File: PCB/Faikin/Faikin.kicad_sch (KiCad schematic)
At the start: 30 parts, among them J1 1x5, J2 TC2030-USB-NL-DS, J3 Reset, Q1 BSS138PS, U2 ESP32-S3-MINI-1, U3 MD8942

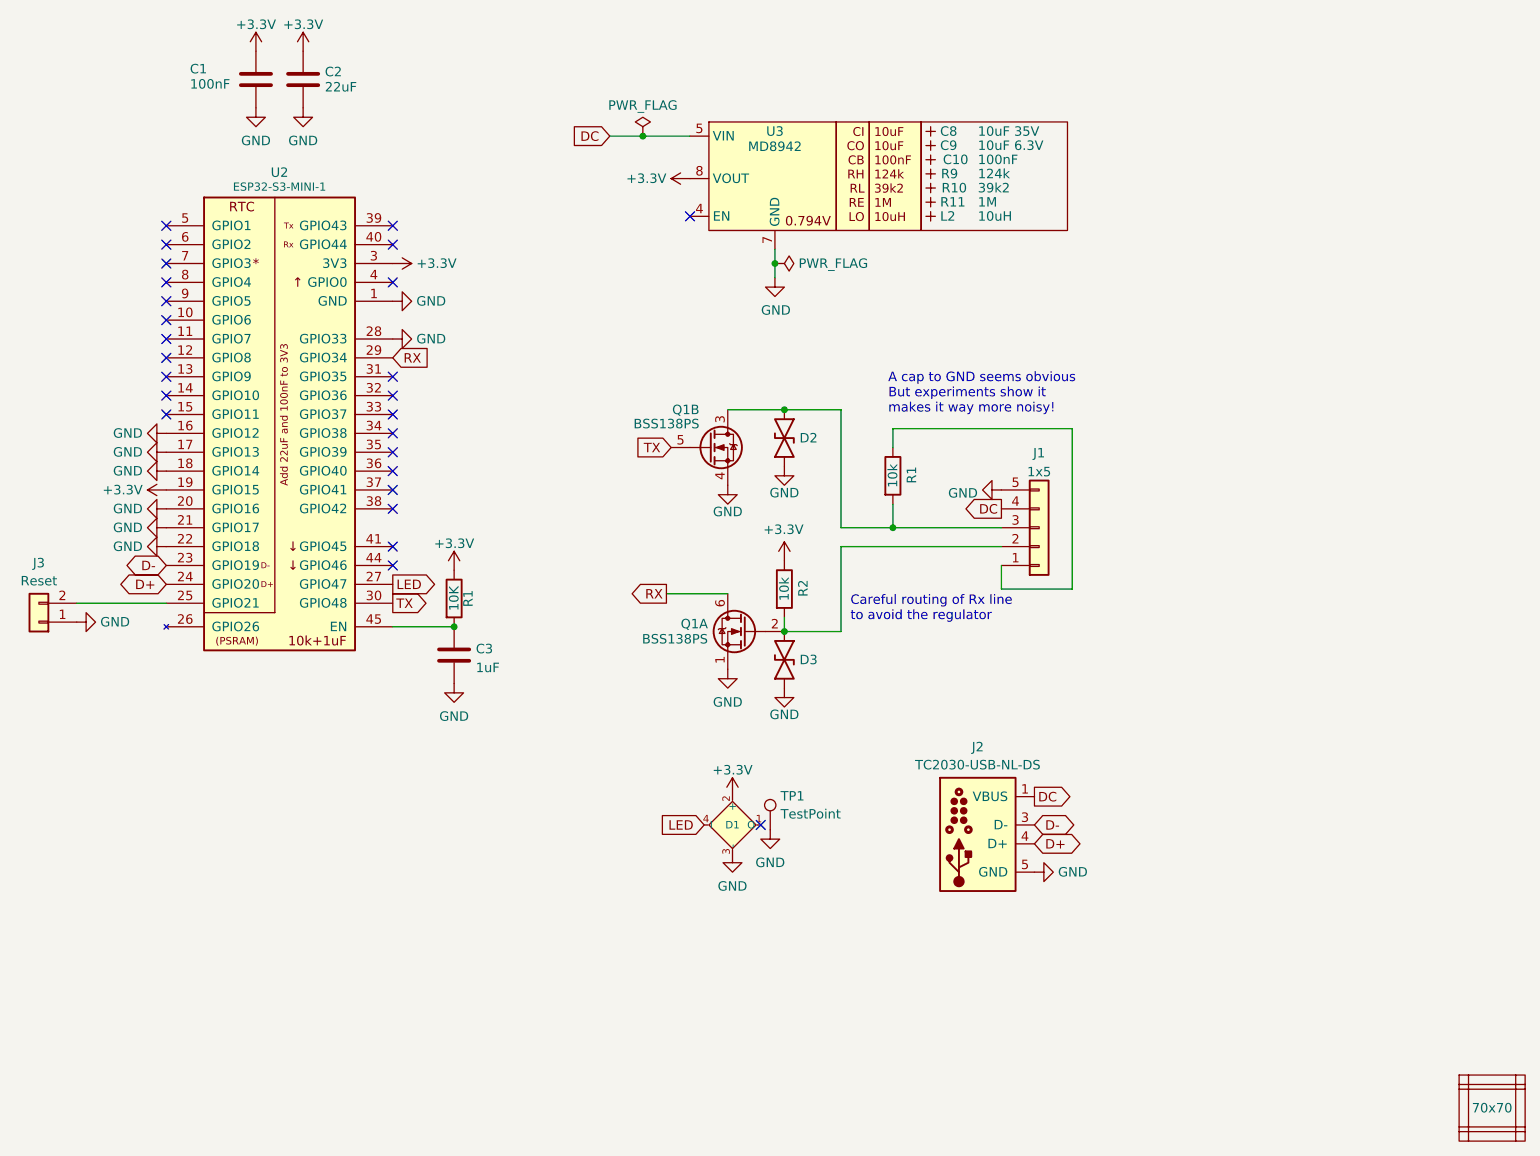
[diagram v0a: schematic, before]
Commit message: Added diode
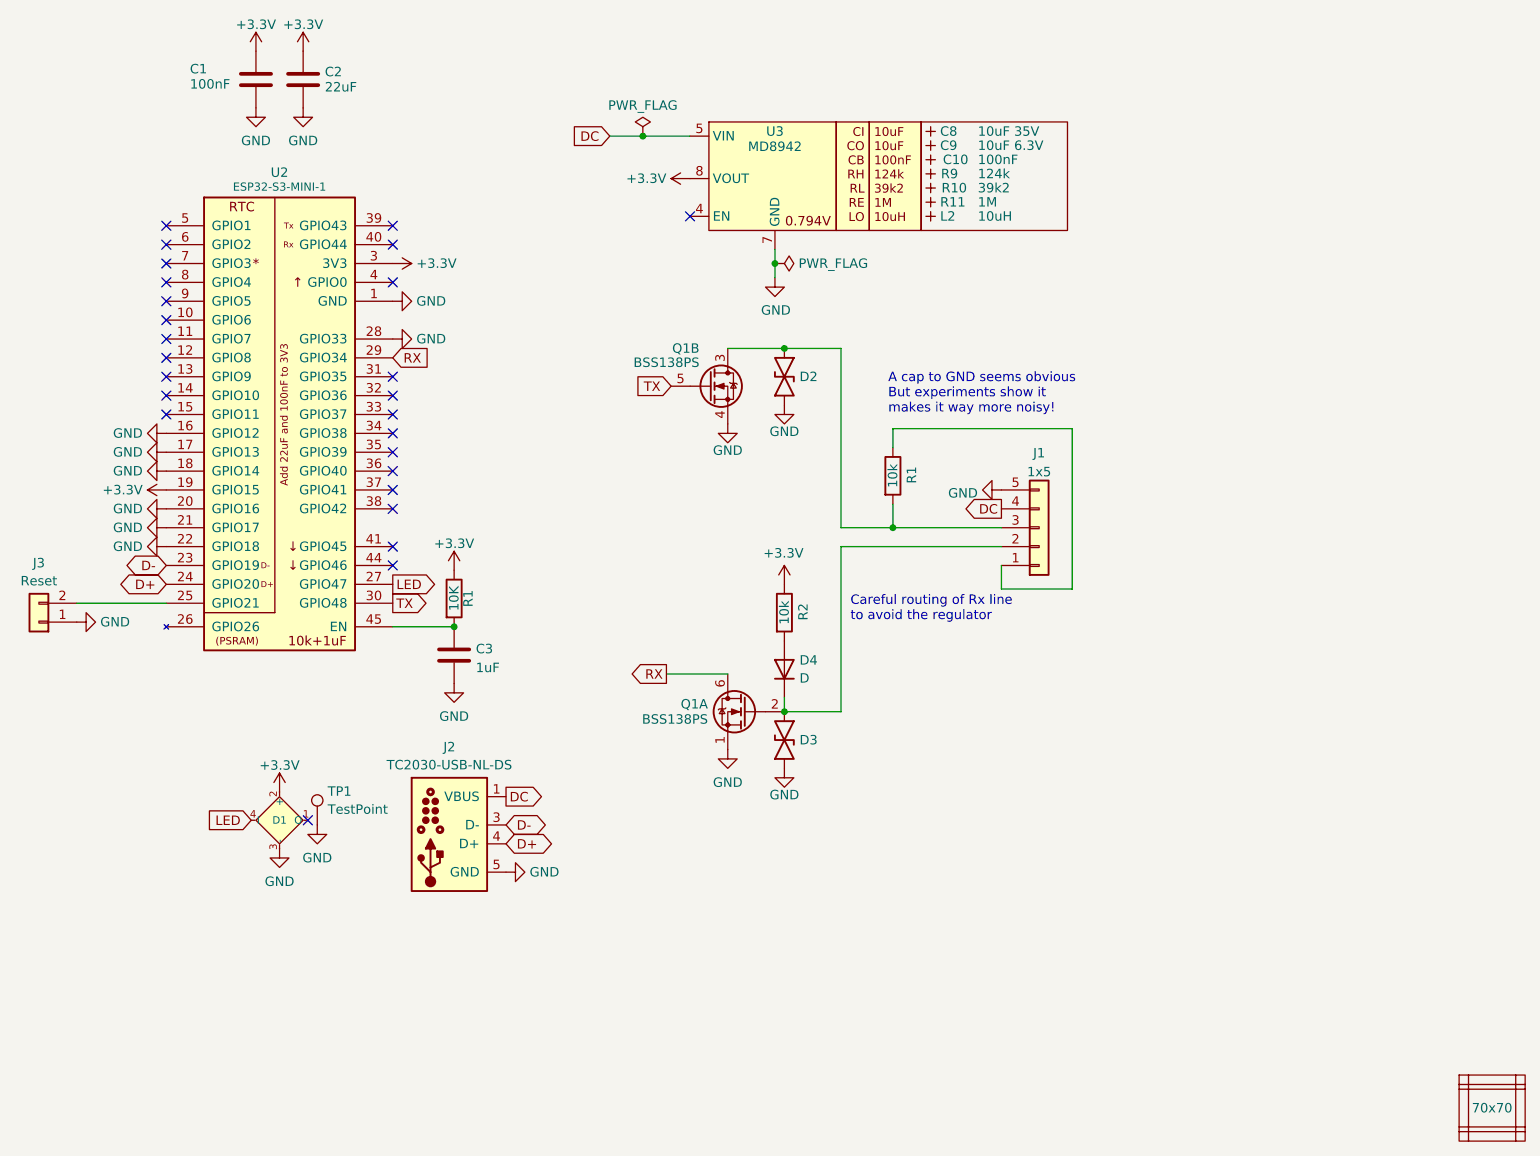
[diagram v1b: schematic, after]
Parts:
- added D4: D, RevK:D_0402, symbol Device:D
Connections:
- net at D3.2, J1.2 (Pin_2), Q1.2 (GN): now also D4.1 (K); no longer R2.2
- new net: D4.2 (A), R2.2
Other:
- moved on the sheet: D1, D2, D3, J2, Q1A, Q1B, R2, TP1
